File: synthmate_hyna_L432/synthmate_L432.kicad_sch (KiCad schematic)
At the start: 54 parts, among them J1 USB_C_synthmate, J2 DIN-5_180degree, J3 USB_C_connector_board, J4 DIN-5_180degree, J5 Conn_01x15, J6 Conn_01x06, J8 Conn_ST_STDC14, SW1 RotaryEncoder_Switch, SW2 SW_Push, SW3 SW_Push, SW4 SW_Slide_DPDT, U1 STM32L432KCUx, U2 TS3USB221ARSER, U3 MIC5365-1.0YC5, U4 TS5A23159RSE, U6 74LV14

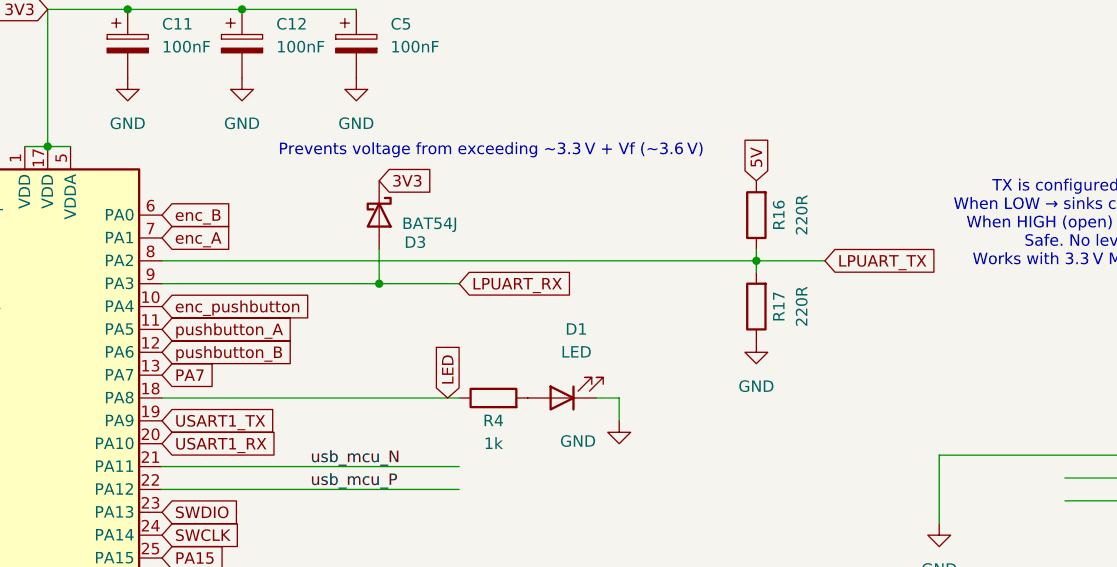
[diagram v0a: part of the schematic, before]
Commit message: cleanup
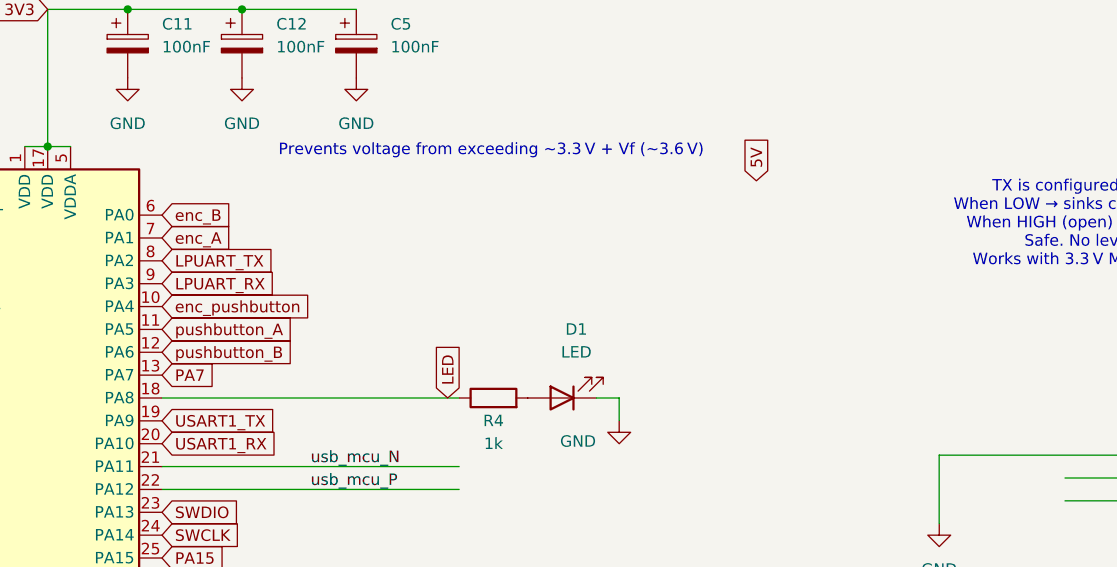
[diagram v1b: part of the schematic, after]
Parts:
- removed D3: BAT54J, Diode_SMD:D_SOD-323F, symbol Diode:BAT54J
- removed R16, R17: 220R, Resistor_SMD:R_0603_1608Metric_Pad0.98x0.95mm_HandSolder, symbol Device:R
